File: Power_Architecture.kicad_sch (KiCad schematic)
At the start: 0 parts

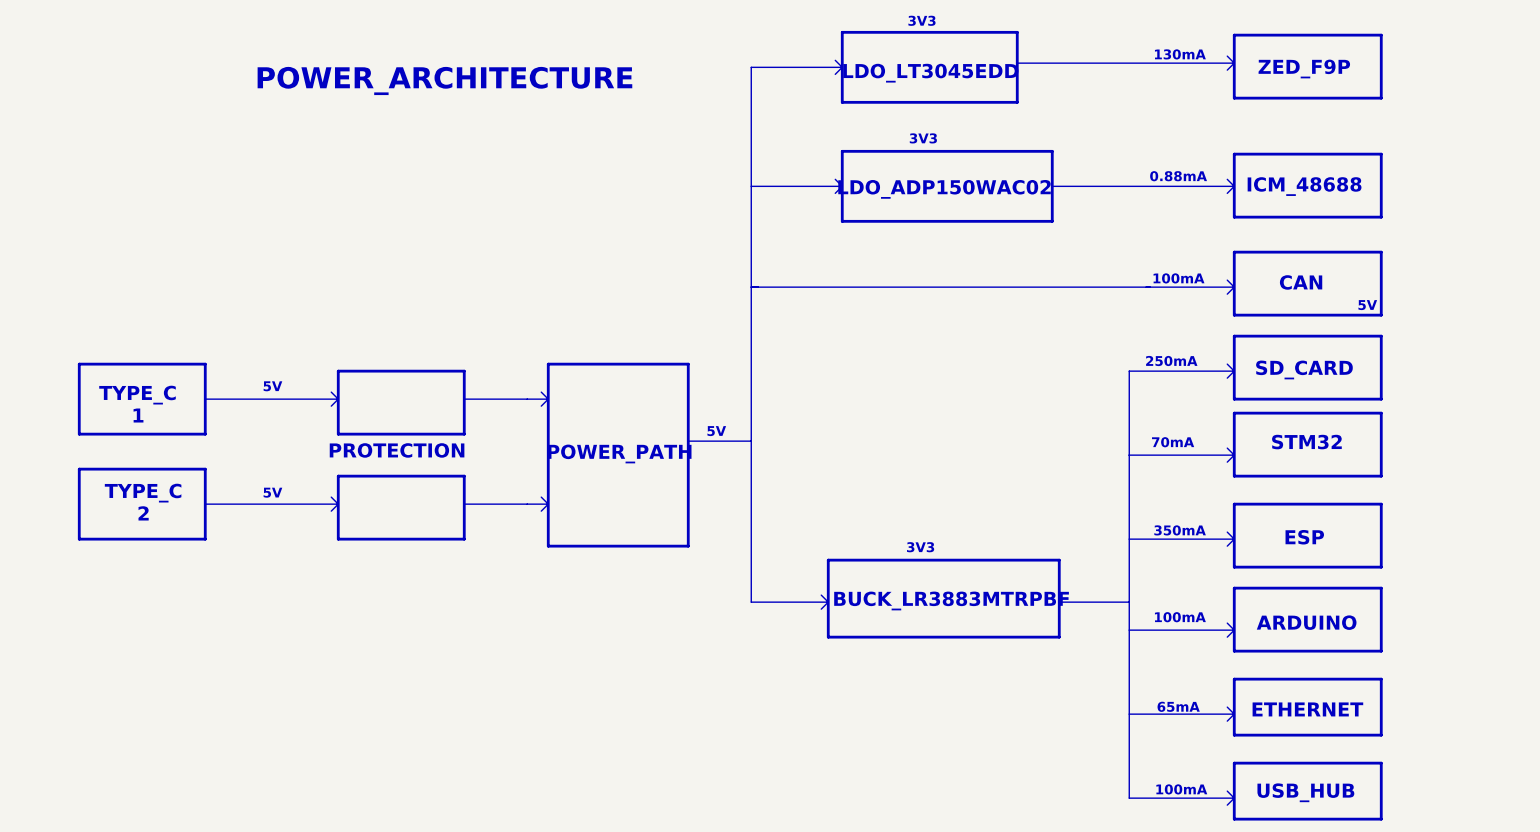
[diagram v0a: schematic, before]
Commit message: 18.09.2026
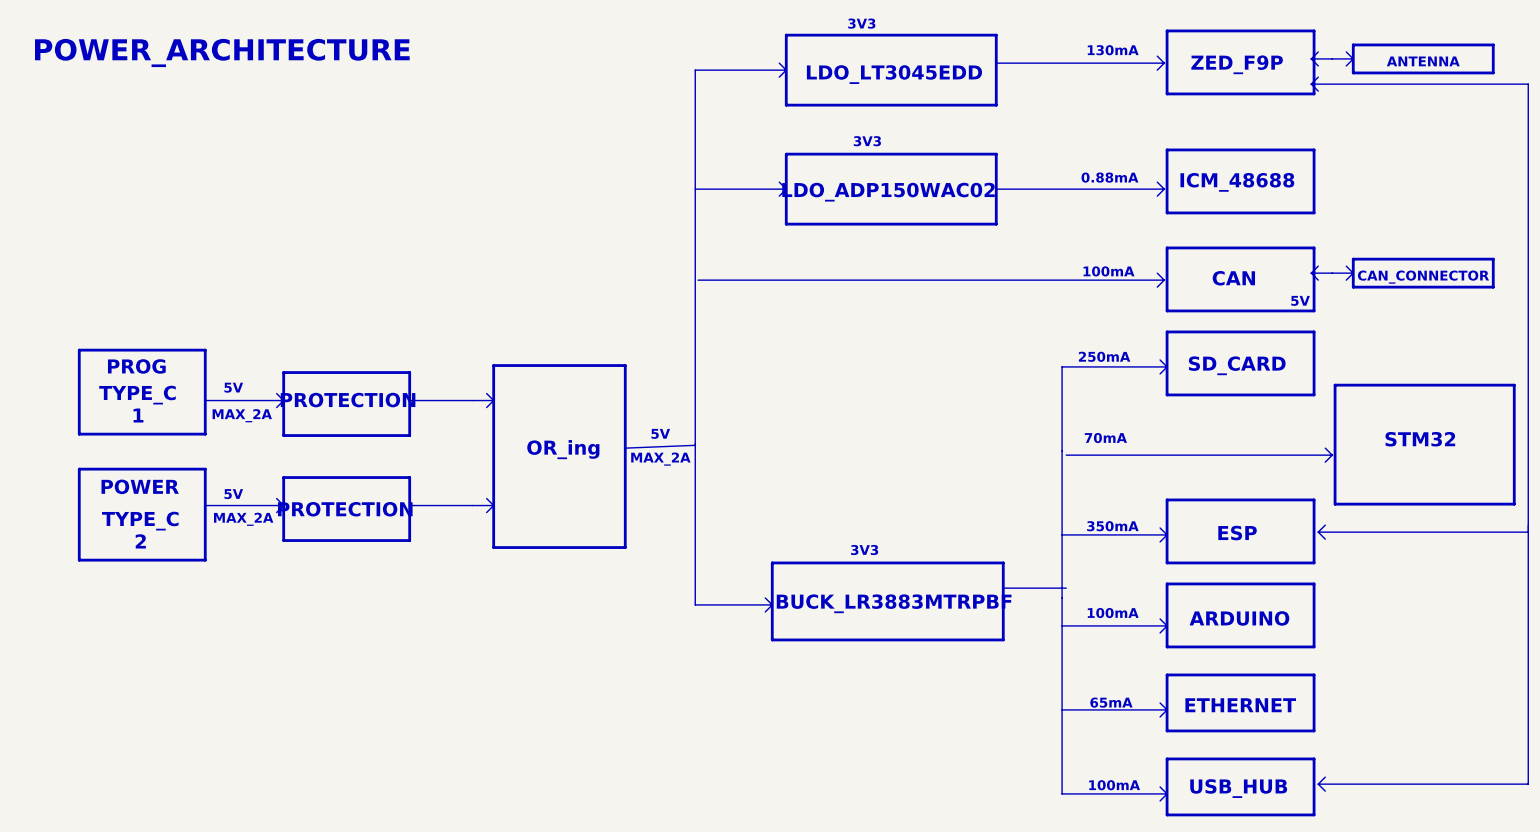
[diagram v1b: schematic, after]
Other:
- note added: "ANTENNA"
- note added: "CAN_CONNECTOR"
- note added: "MAX_2A"
- note added: "OR_ing"
- note added: "POWER"
- note added: "PROG"
- note removed: "POWER_PATH"
